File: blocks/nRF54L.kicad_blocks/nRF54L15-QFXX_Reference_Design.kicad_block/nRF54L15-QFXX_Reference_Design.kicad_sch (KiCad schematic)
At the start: 21 parts, among them U1 nRF54L15-QFXX, Y1 32MHz

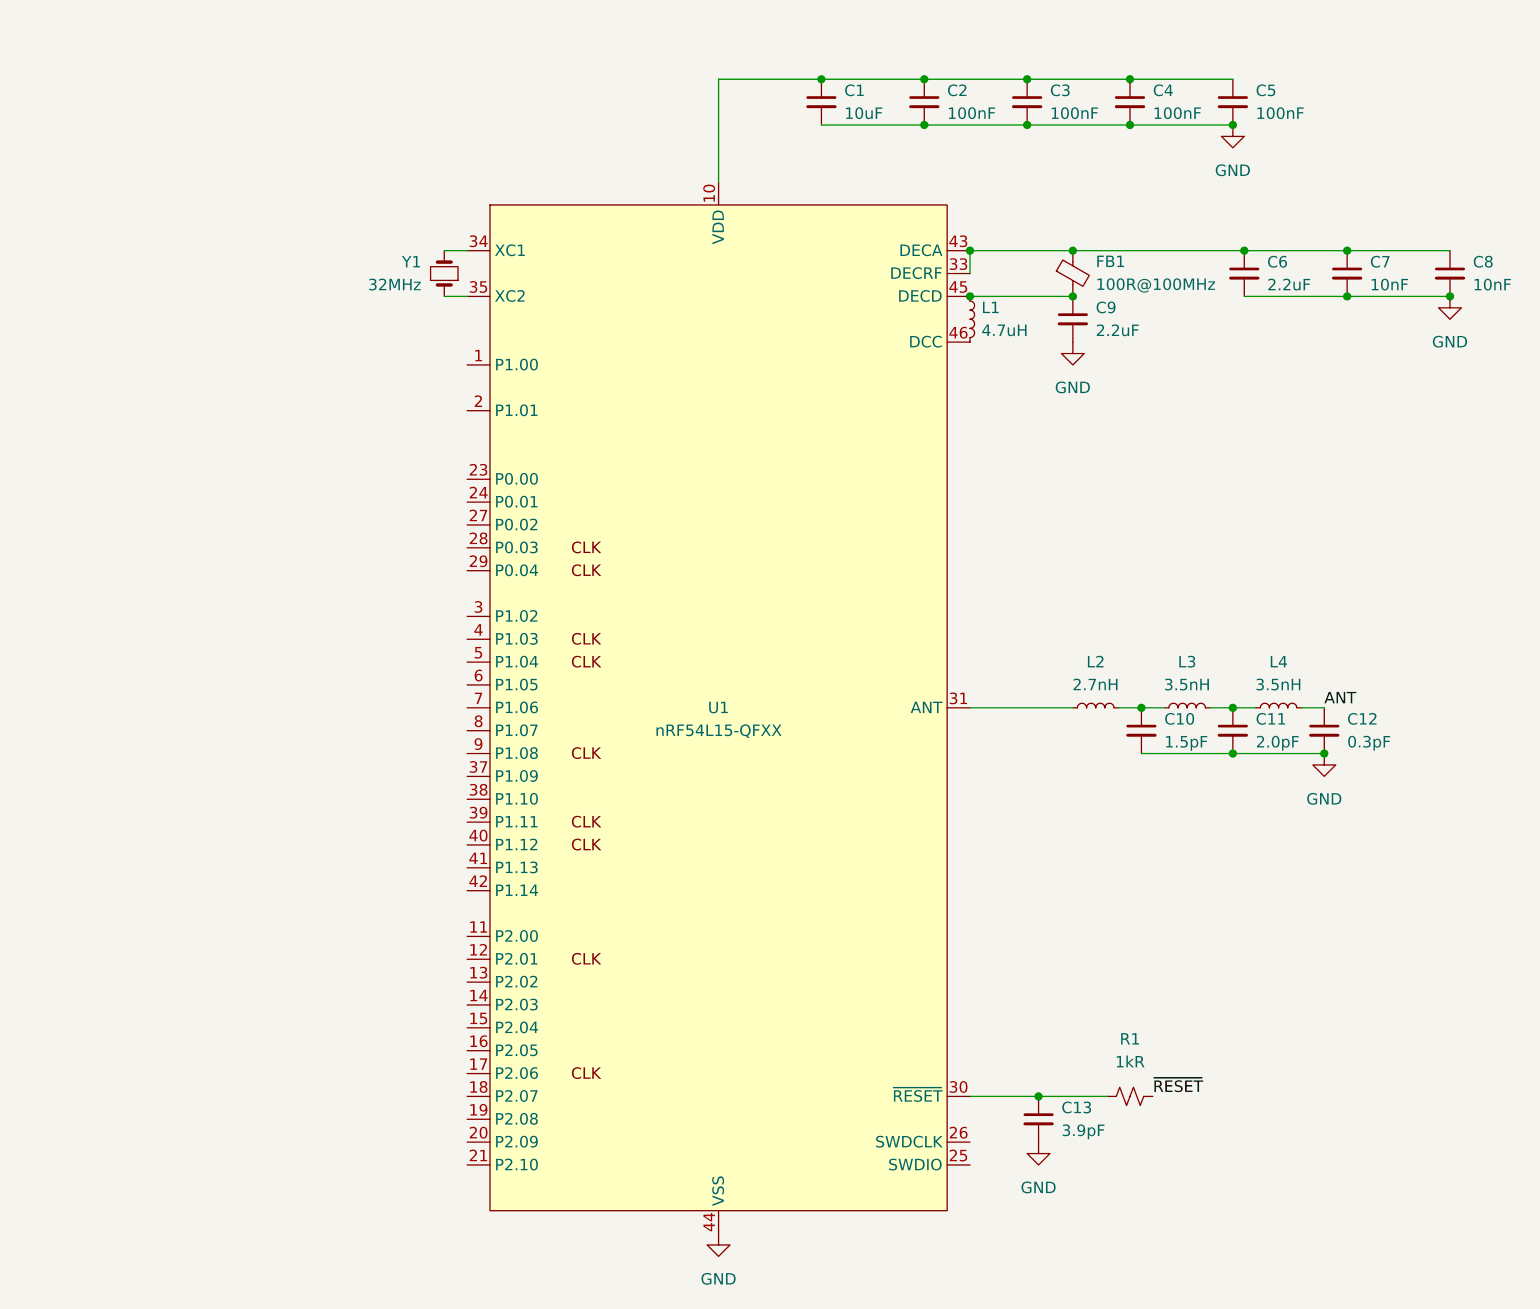
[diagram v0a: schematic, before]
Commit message: updates for ref design test
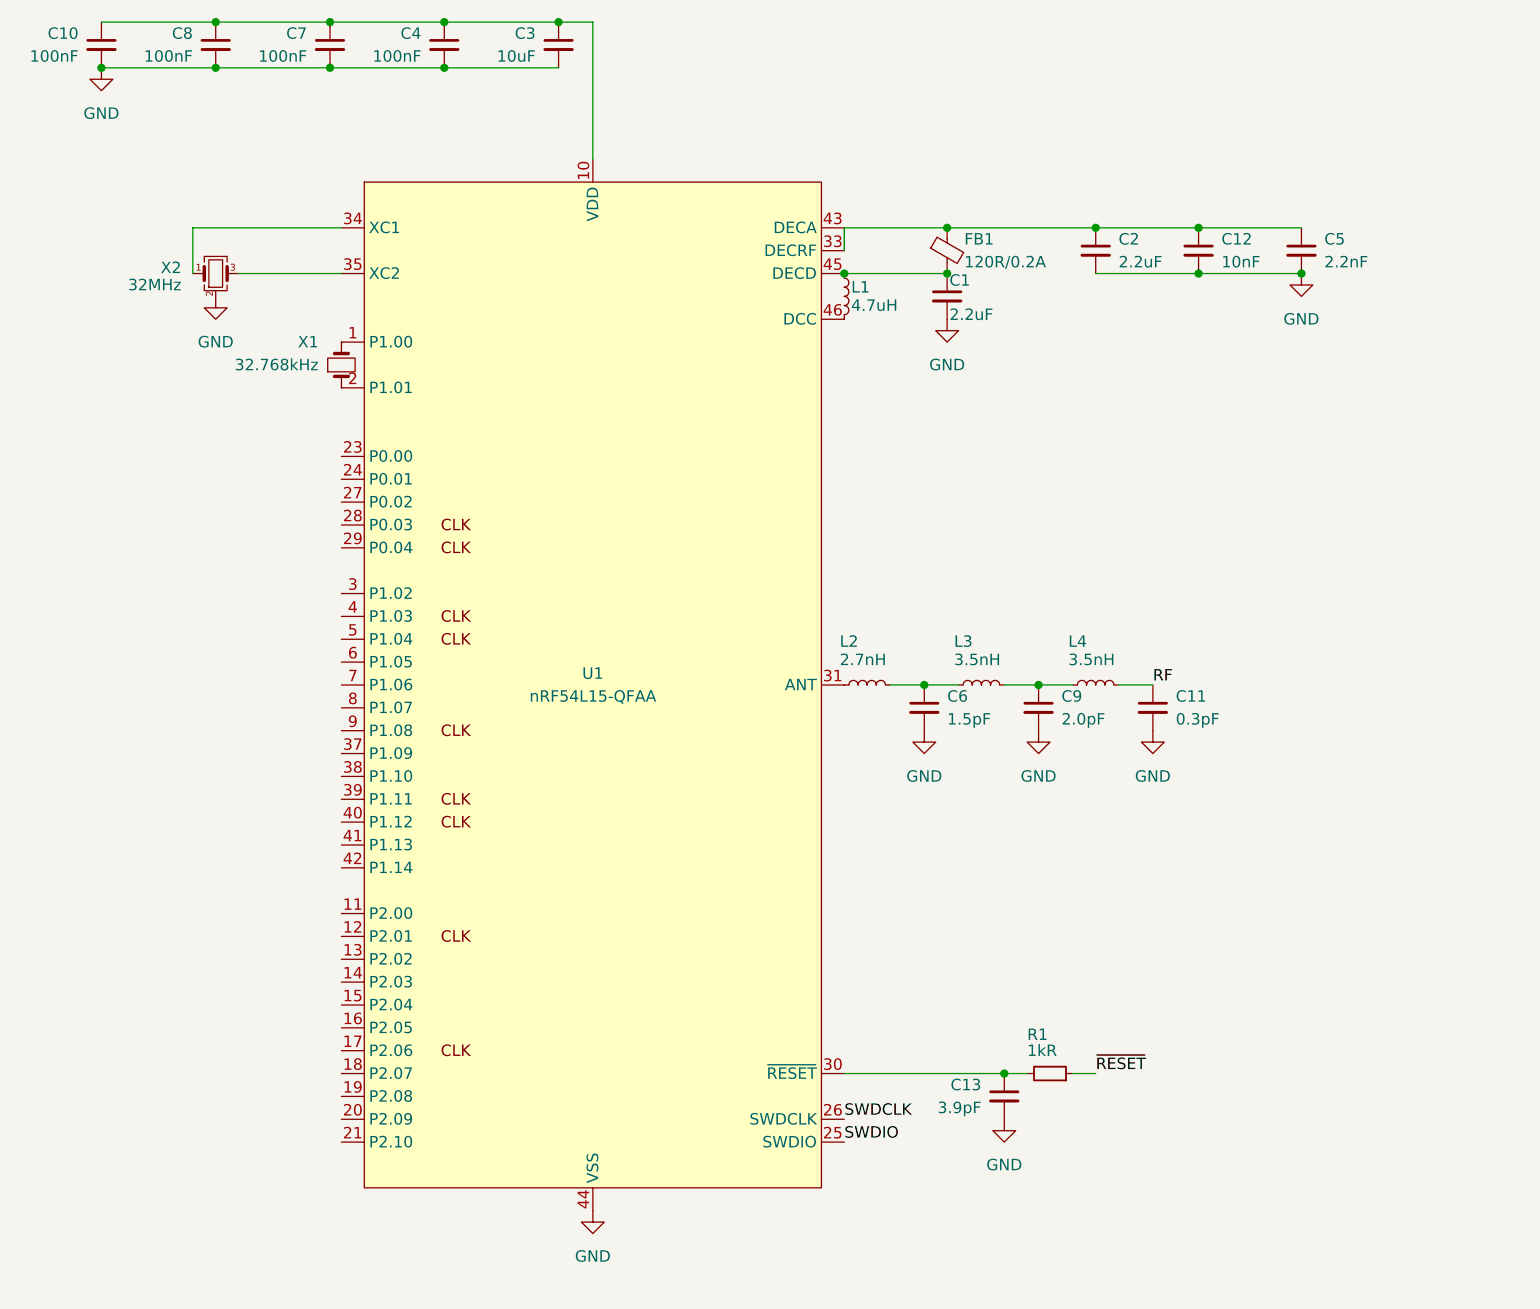
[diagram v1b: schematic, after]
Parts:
- removed R1: 1kR, symbol Device:R_Small_US
- removed Y1: 32MHz, symbol Device:Crystal_Small
- added R1: 1kR, passives:R_0201_0603Metric_L, symbol Device:R_Small
- added X1: 32.768kHz, Crystal:Crystal_SMD_2012-2Pin_2.0x1.2mm, symbol Device:Crystal_Small
- added X2: 32MHz, Crystal:Crystal_SMD_2016-4Pin_2.0x1.6mm, symbol Device:Crystal_GND24_Small
- C1: value 10uF -> 2.2uF; footprint (none) -> passives:C_0201_0603Metric_L
- C10: value 1.5pF -> 100nF; footprint (none) -> passives:C_0201_0603Metric_L
- C11: value 2.0pF -> 0.3pF; footprint (none) -> passives:C_0201_0603Metric_L
- C12: value 0.3pF -> 10nF; footprint (none) -> passives:C_0201_0603Metric_L
- C13, C4: footprint (none) -> passives:C_0201_0603Metric_L
- C2: value 100nF -> 2.2uF; footprint (none) -> passives:C_0201_0603Metric_L
- C3: value 100nF -> 10uF; footprint (none) -> passives:C_0402_1005Metric_L
- C5: value 100nF -> 2.2nF; footprint (none) -> passives:C_0201_0603Metric_L
- C6: value 2.2uF -> 1.5pF; footprint (none) -> passives:C_0201_0603Metric_L
- C7, C8: value 10nF -> 100nF; footprint (none) -> passives:C_0201_0603Metric_L
- C9: value 2.2uF -> 2.0pF; footprint (none) -> passives:C_0201_0603Metric_L
- FB1: value 100R@100MHz -> 120R/0.2A; footprint (none) -> passives:L_0201_0603Metric_L
- L1: footprint (none) -> passives:L_0603_1608Metric_L
- L2, L3, L4: footprint (none) -> passives:L_0201_0603Metric_L
- U1: value nRF54L15-QFXX -> nRF54L15-QFAA; footprint Package_DFN_QFN:QFN-48-1EP_6x6mm_P0.4mm_EP4.6x4.6mm -> Package_DFN_QFN:QFN-48-1EP_6x6mm_P0.4mm_EP4.6x4.6mm_ThermalVias
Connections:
- net GND: now also X2.2 (G), X2.4 (G)
- net ~{RESET}: now also R1.1
- net at C13.1, U1.30 (~{RESET}): now also R1.2
- net at FB1.1, U1.33 (DECRF), U1.43 (DECA): now also C12.1, C2.1, C5.1; no longer C6.1, C7.1, C8.1
- net at FB1.2, L1.1, U1.45 (DECD): now also C1.1; no longer C9.1
- net at C3.1, C4.1, U1.10 (VDD)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: now also C10.1, C7.1, C8.1; no longer C1.1, C2.1, C5.1
- net at U1.35 (XC2): now also X2.3
- net at U1.34 (XC1): now also X2.1
- net at L3.2, L4.1: now also C9.1; no longer C11.1
- net at L2.2, L3.1: now also C6.1; no longer C10.1
- net at U1.1 (P1.00): now also X1.2
- net at U1.2 (P1.01): now also X1.1
- net SWDIO: now reaches U1.25 (SWDIO)
- net SWDCLK: now reaches U1.26 (SWDCLK)
- net ANT renamed RF
- net RF: now also C11.1; no longer C12.1
